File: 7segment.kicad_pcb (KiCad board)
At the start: 2 copper layers, 62.9 x 22.9 mm, 21 parts, among them J1 RESET, J2 IN_UP, J3 VCC, J4 IN_DOWN, J5 GND, J6 LATCH, J7 LATCH, U1 LTD-2601G, U2 ATmega8535-16AU, U3 LTD-2601G, U4 LTD-2601G

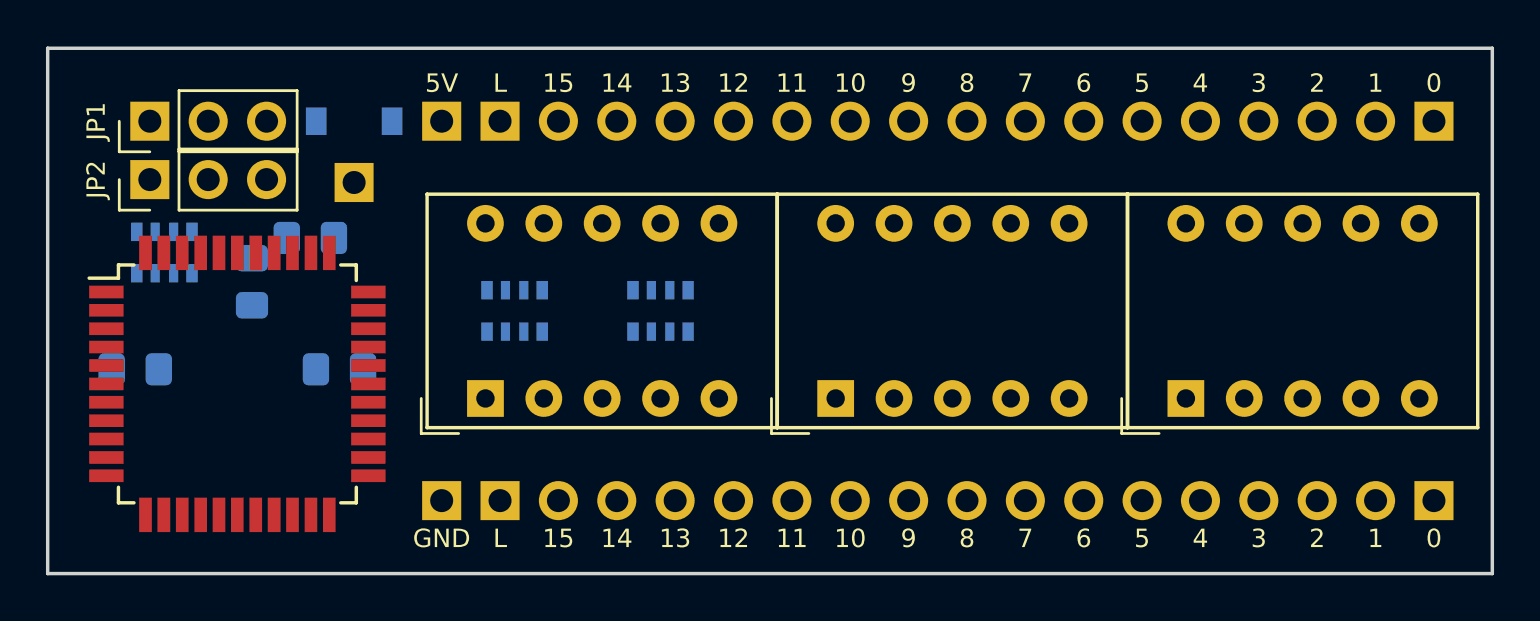
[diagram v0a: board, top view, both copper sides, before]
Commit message: Routing
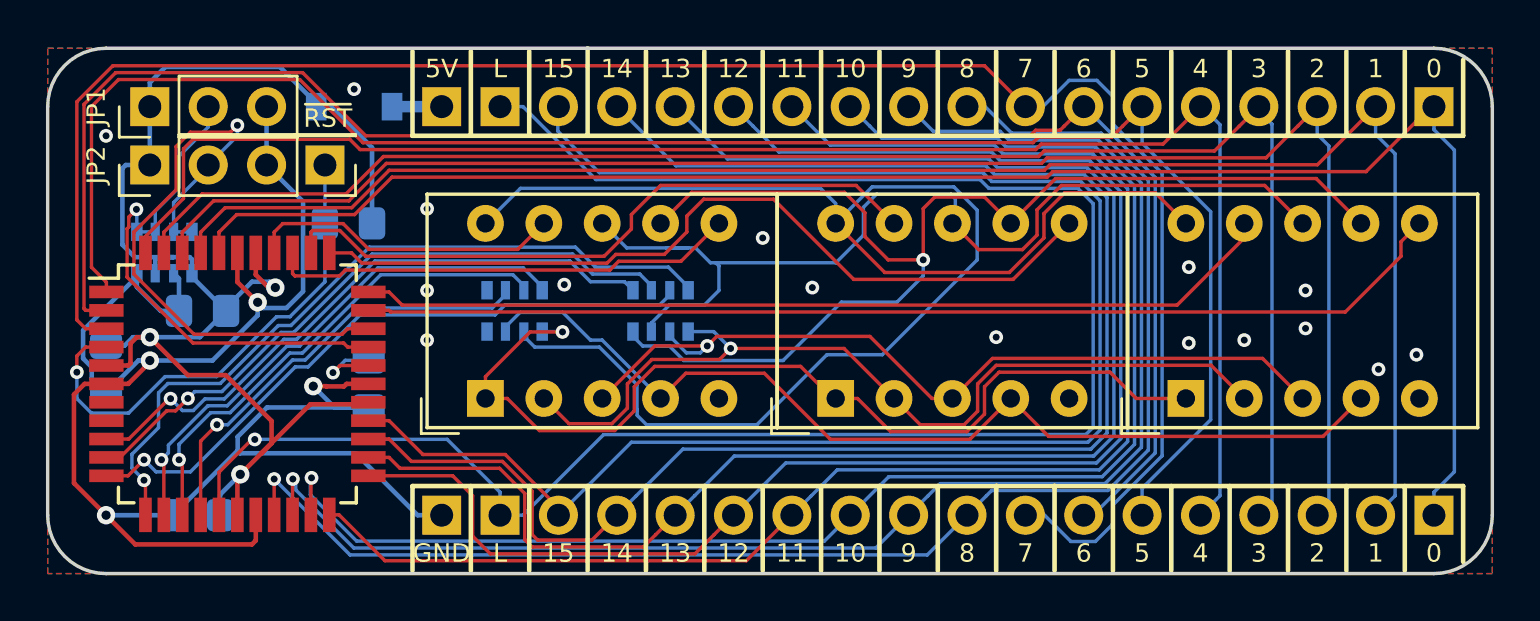
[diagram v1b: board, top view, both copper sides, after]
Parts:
- added C4: 0.1uF, Capacitor_SMD:C_0805_2012Metric_Pad1.15x1.40mm_HandSolder, B.Cu at (45.8, 55.9)
- J1: moved to F.Cu
- moved C1 2.50 mm to (46.1, 47.0), turned to 180 degrees
- moved R3 1.78 mm to (52.5, 43.2), turned to 180 degrees
- moved J1 1.48 mm to (51.4, 40.6), turned to 180 degrees
- moved C3 1.42 mm to (53.3, 50.2), turned to 90 degrees
- moved C2 1.27 mm to (41.9, 49.5), turned to 270 degrees
- moved J4 0.64 mm to (99.7, 55.9)
- moved J5 0.64 mm to (56.5, 55.9)
- moved J6 0.64 mm to (59.1, 55.9)
- moved D1 0.63 mm to (52.7, 38.1)
- moved J2 0.63 mm to (99.7, 38.1)
- moved J3 0.63 mm to (56.5, 38.1)
- moved J7 0.63 mm to (59.1, 38.1)
- moved JP1 0.63 mm to (43.8, 38.1)
- moved JP2 0.63 mm to (43.8, 40.6)
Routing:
- net SCK: track 0.00 -> 83.1 mm
- net Net-(J6-Pad1): track 0.00 -> 81.3 mm, vias 0 -> 1
- net GND: track 0.00 -> 80.4 mm, vias 0 -> 20
- net MOSI: track 0.00 -> 76.6 mm
- net MISO: track 0.00 -> 76.2 mm
- net /IN0: track 0.00 -> 74.6 mm
- net /IN1: track 0.00 -> 72.8 mm
- net /IN15: track 0.00 -> 71.2 mm
- net /IN2: track 0.00 -> 70.8 mm
- net SEG_F: track 0.00 -> 70.4 mm
- net /IN14: track 0.00 -> 70.2 mm
- net /IN4: track 0.00 -> 69.1 mm
- net /IN3: track 0.00 -> 69.1 mm
- net /IN13: track 0.00 -> 68.4 mm
- net /IN12: track 0.00 -> 66.4 mm
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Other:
- outline, holes or cut-outs redrawn
- net class VIN added: clearance 0.2, trace_width 0.5, via_dia 0.6, via_drill 0.3
- board text added: "16 bit DEC/HEX Display RevA 2019 Dominic Thibodeau dev@hotkeysoft.net"
- board text added: "JP1: DEC/HEX"
- board text added: "JP2: LATCH"
- board text added: "LATCH L->H LATCH H->L NOT LATCHED"
- board text added: "POS"
- board text removed: "DECIMAL/HEX"
- board text removed: "JP1"
- board text removed: "RevB 2019 dev@hotkeysoft.net"
